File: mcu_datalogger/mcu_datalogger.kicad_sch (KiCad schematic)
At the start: 25 parts, among them U1 24LC1025, U2 24LC1025, U3 DS1337S_, U4 ATMEGA328P-AU, Y1 32.768 KHz, Y2 16 MHz

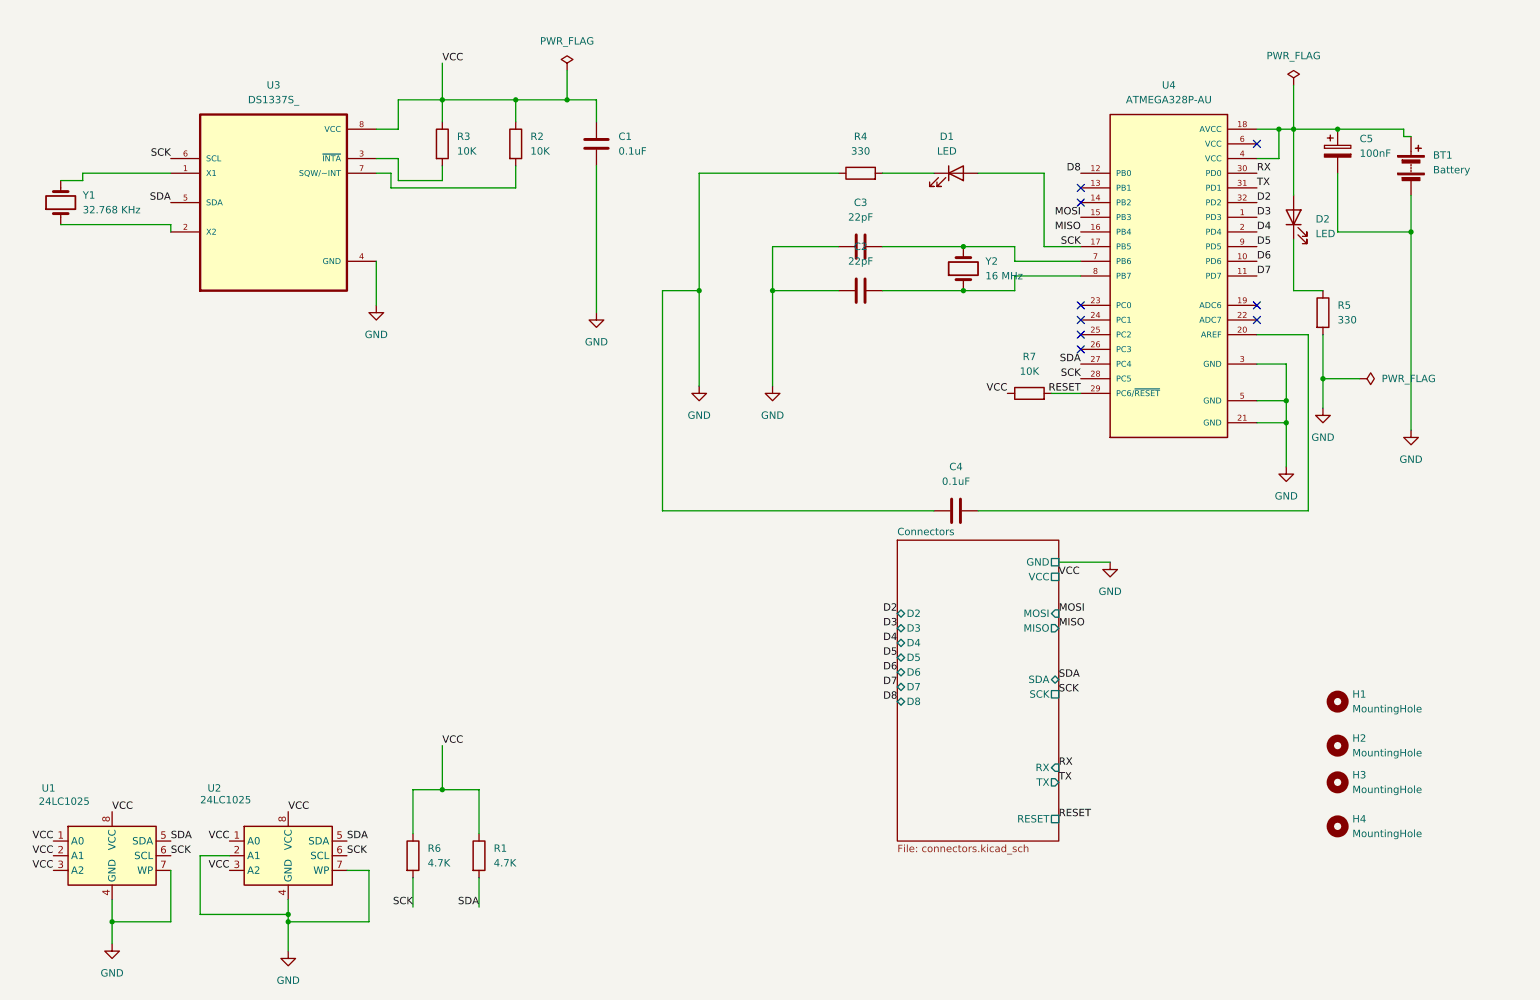
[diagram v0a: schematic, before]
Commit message: add comments
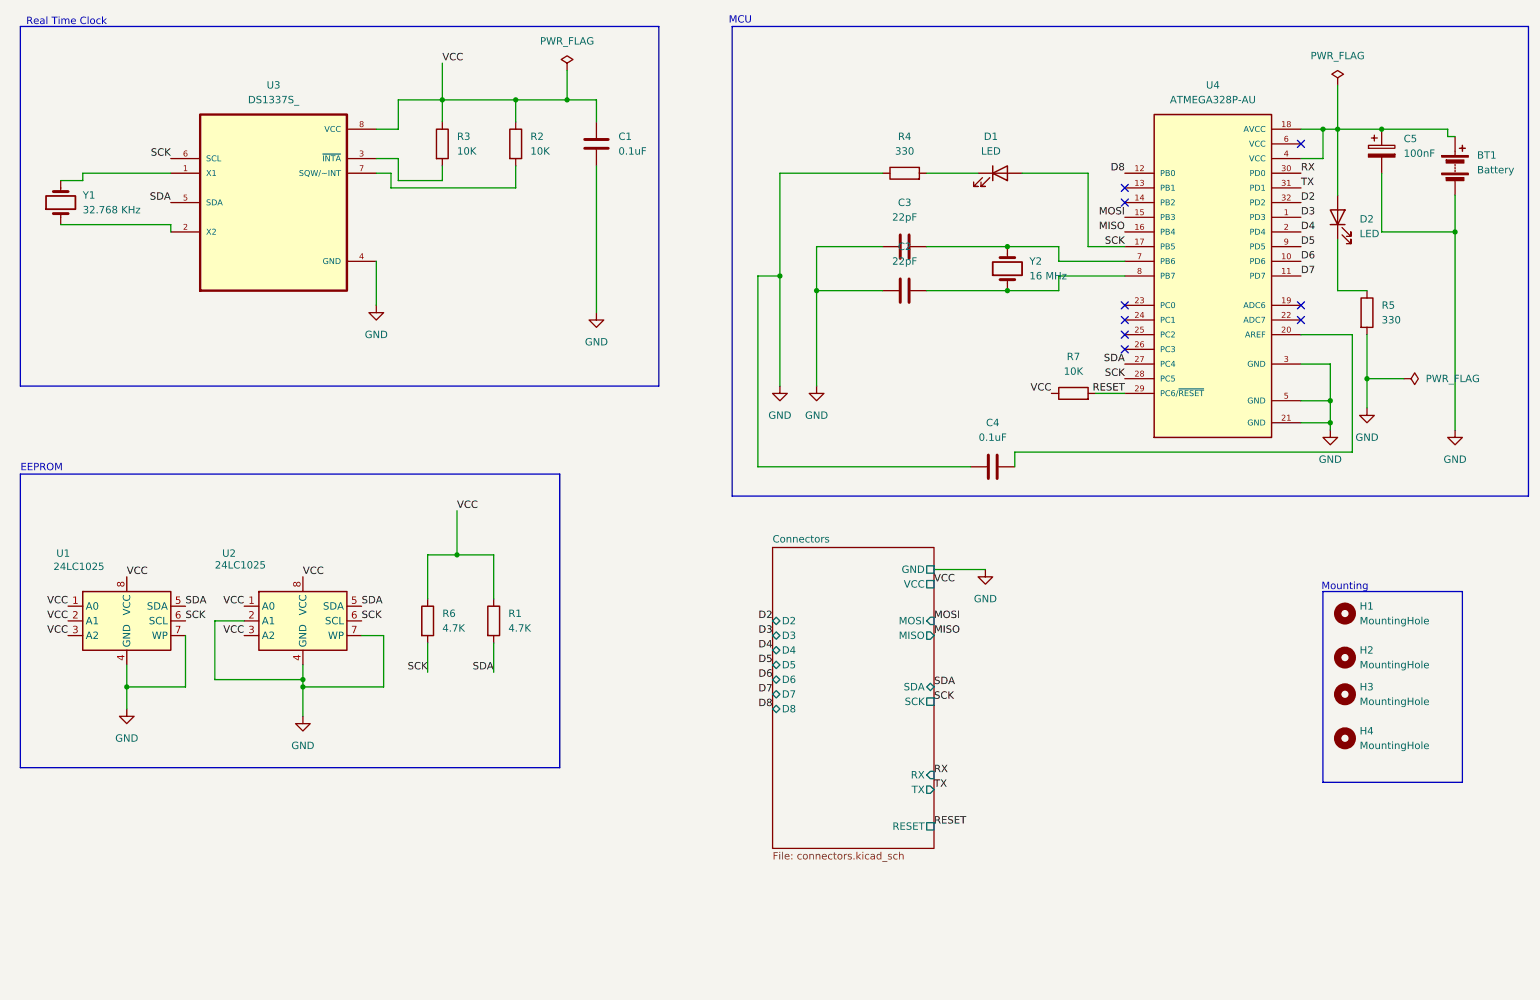
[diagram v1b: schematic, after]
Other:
- note added: "EEPROM"
- note added: "MCU"
- note added: "Mounting"
- note added: "Real Time Clock"
- moved on the sheet: BT1, C2, C3, C4, C5, D1, D2, H1, H2, H3, H4, R1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
